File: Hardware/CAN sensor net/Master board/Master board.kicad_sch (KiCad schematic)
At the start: 37 parts, among them SW1 SW_Push, SW2 SW_SPDT, U1 STM32F405RGTx, U5 SN65HVD230, U6 SN65HVD230, Y1 16MHz

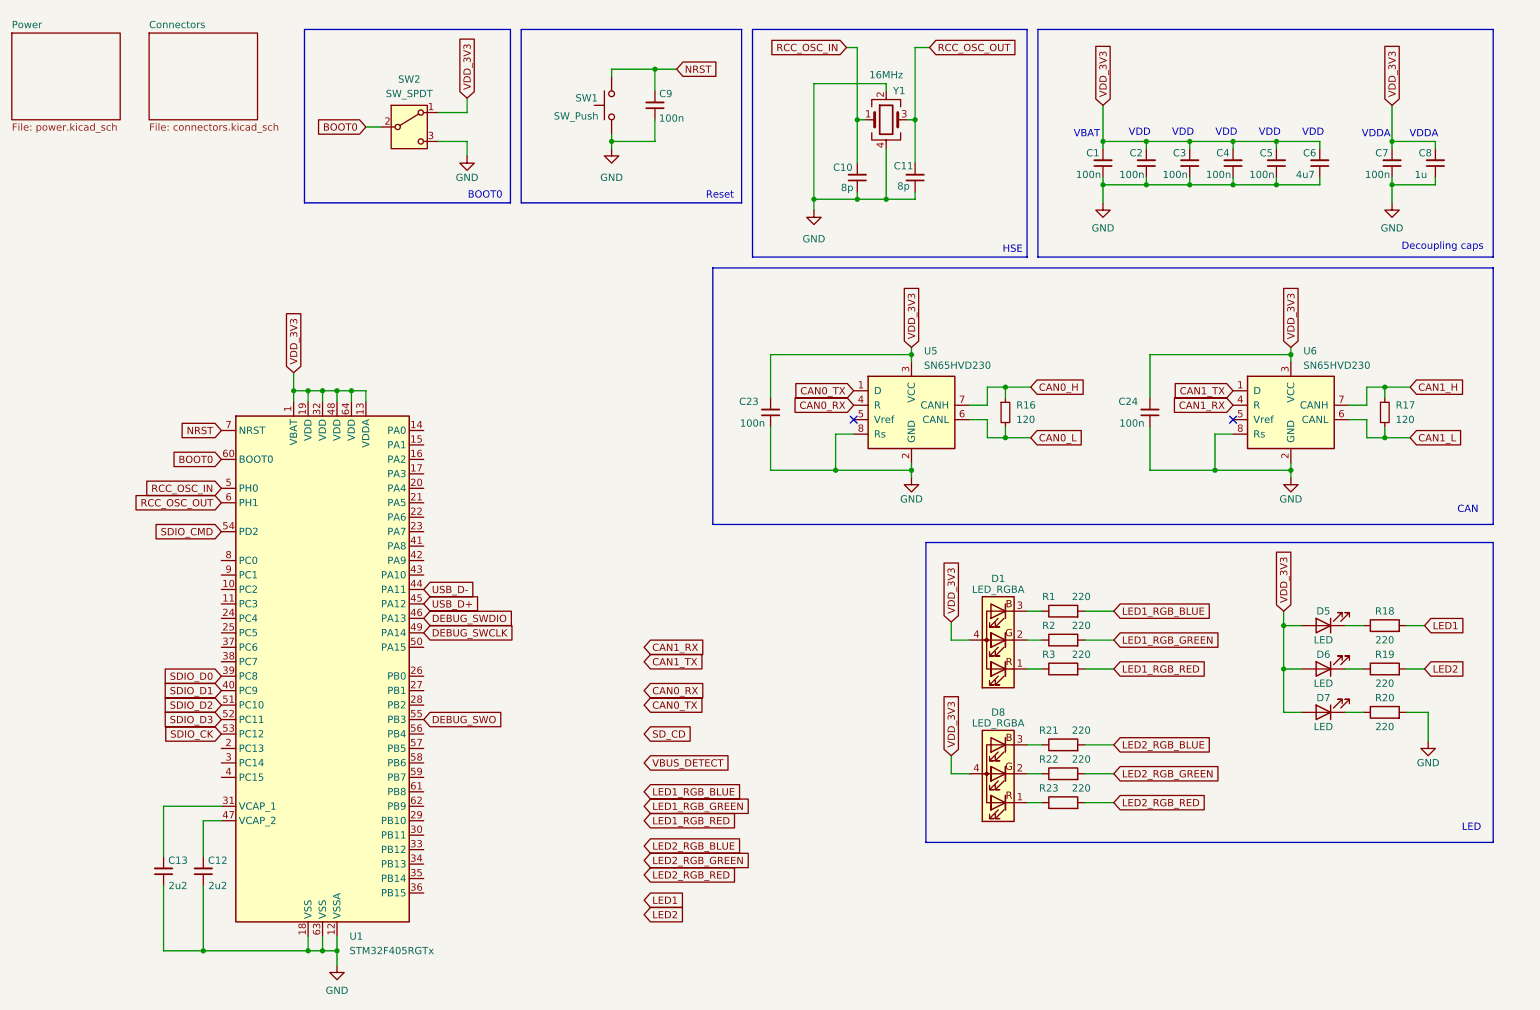
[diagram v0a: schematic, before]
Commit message: added spi flash memory
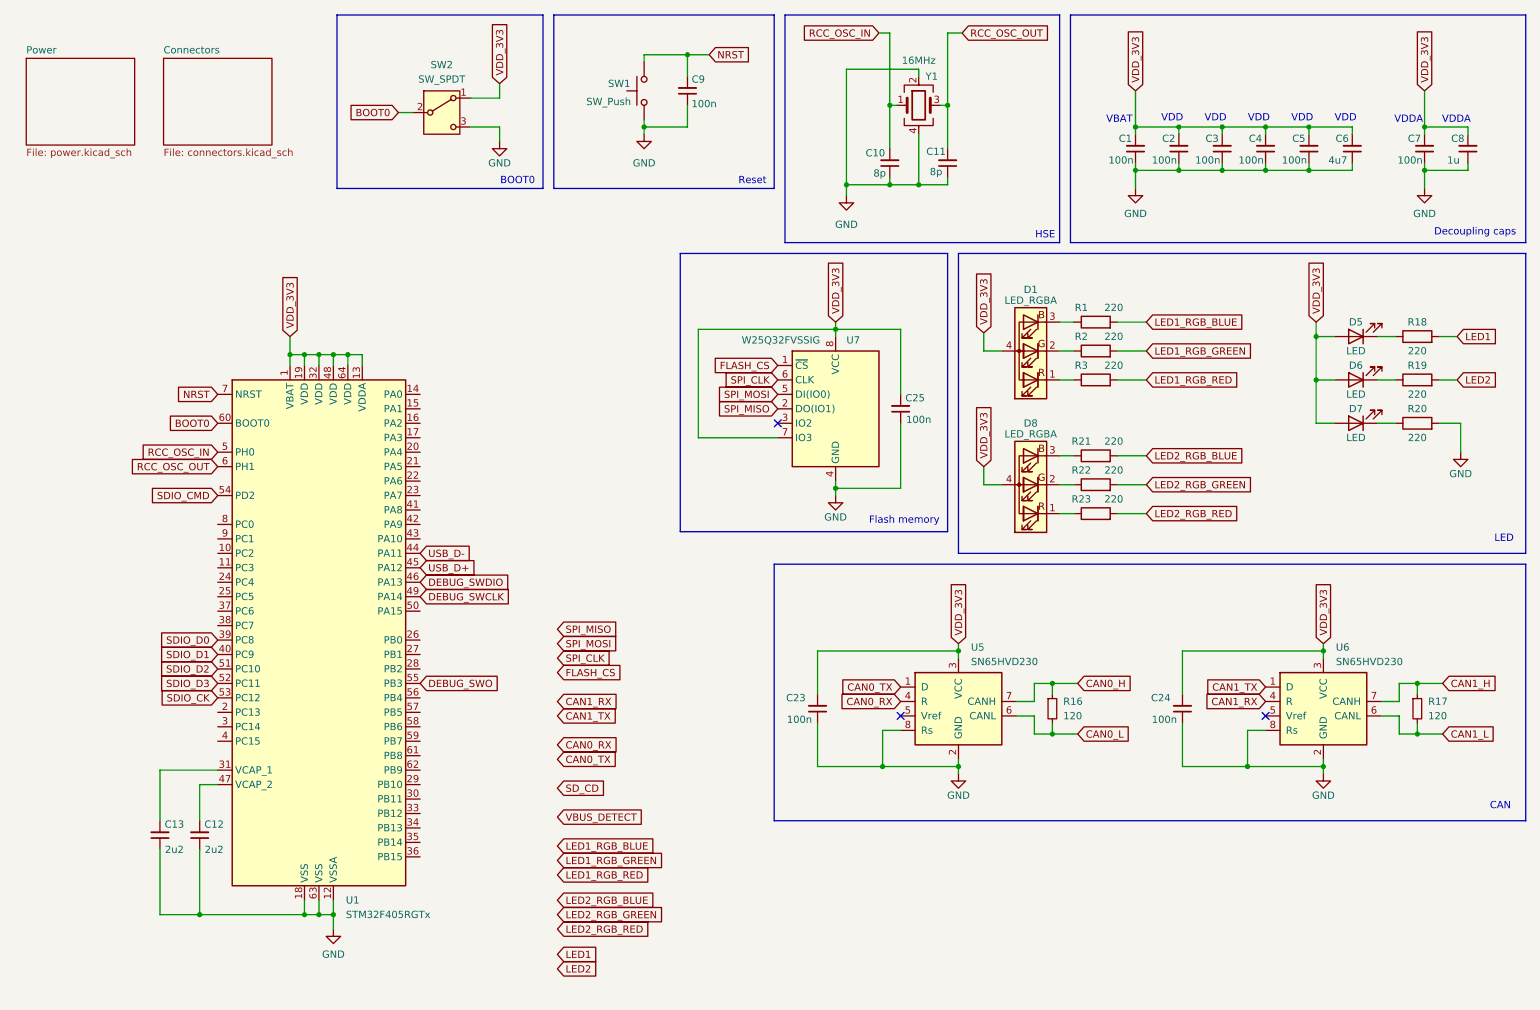
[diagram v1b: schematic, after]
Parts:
- added C25: 100n, Capacitor_SMD:C_0603_1608Metric, symbol Device:C_Small
- added U7: W25Q32FVSSIG, Package_SO:SOIC-8_5.23x5.23mm_P1.27mm, symbol Memory_Flash:W25Q32JVSS
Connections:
- net GND: now also C25.1, U7.4 (GND)
- net VDD_3V3: now also C25.2, U7.7 (IO3), U7.8 (VCC)
- new net FLASH_CS: U7.1 (~{CS})
- new net SPI_CLK: U7.6 (CLK)
- new net SPI_MISO: U7.2 (DO(IO1))
- new net SPI_MOSI: U7.5 (DI(IO0))
- no-connect marks 2 -> 3
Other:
- note added: "Flash memory"
- moved on the sheet: C1, C10, C11, C12, C13, C2, C23, C24, C3, C4, C5, C6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

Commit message: Bugfix
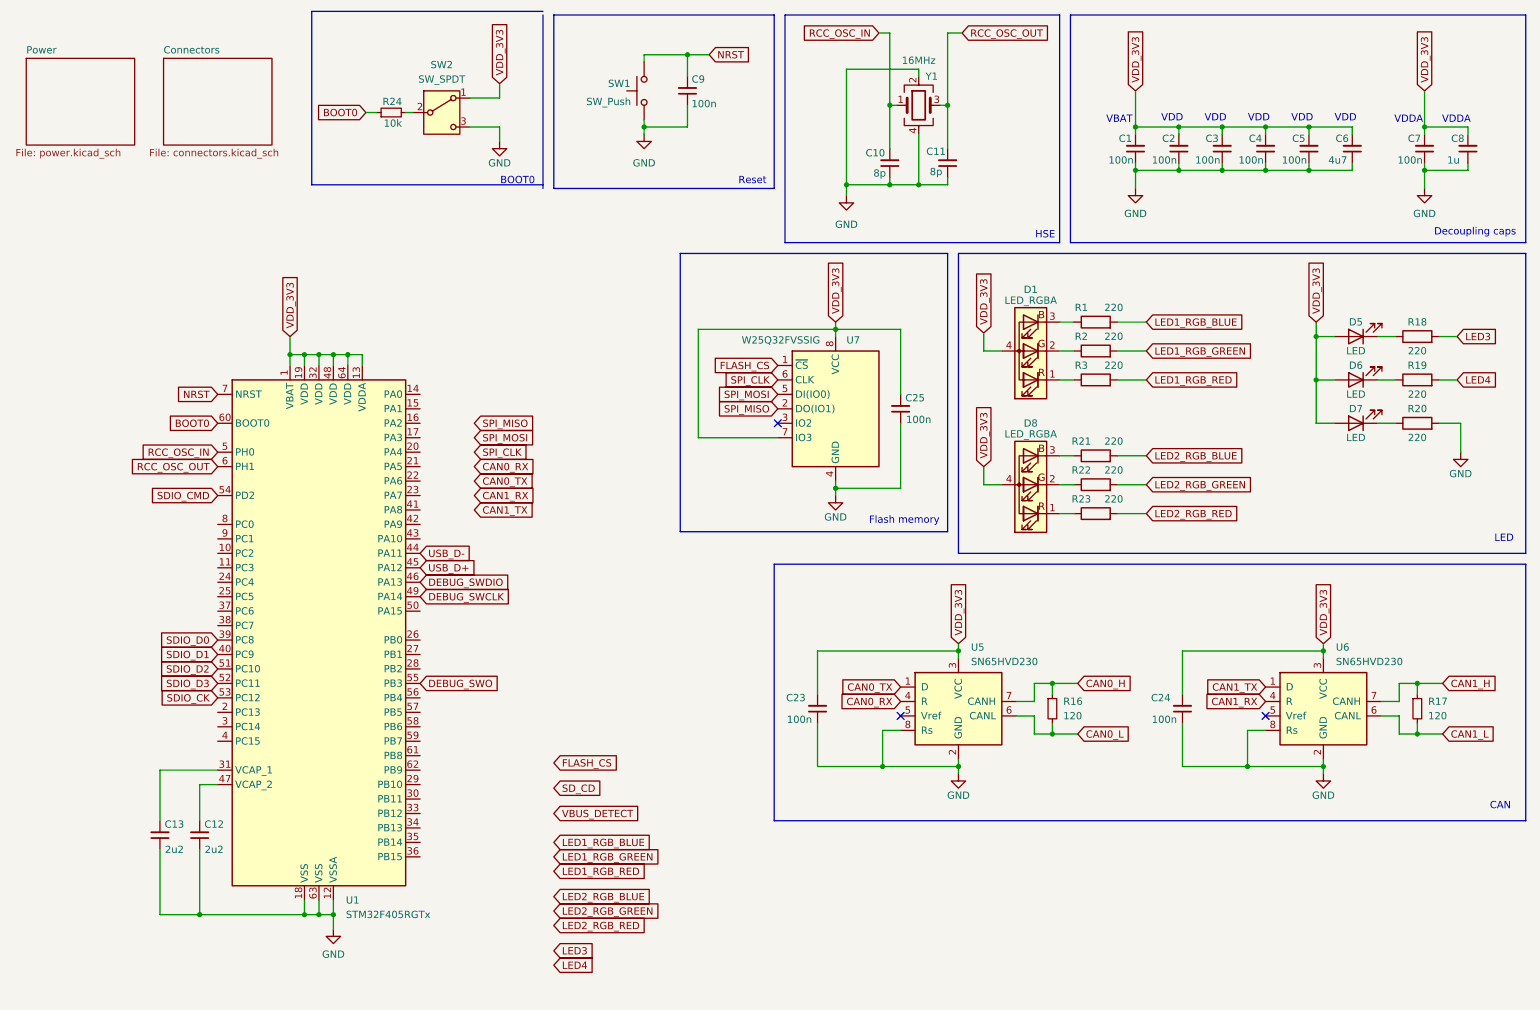
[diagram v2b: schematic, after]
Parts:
- added R24: 10k, Resistor_SMD:R_0603_1608Metric, symbol Device:R_Small
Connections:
- net BOOT0: now also R24.1; no longer SW2.2 (B)
- net LED1 renamed LED3
- net LED2 renamed LED4
- new net: R24.2, SW2.2 (B)
